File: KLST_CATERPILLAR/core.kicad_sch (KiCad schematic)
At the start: 34 parts, among them SW1 BUTTON_RESET, SW2 BUTTON_BOOT_FLASH, U2 STM32H723ZGTx, Y1 16MHz

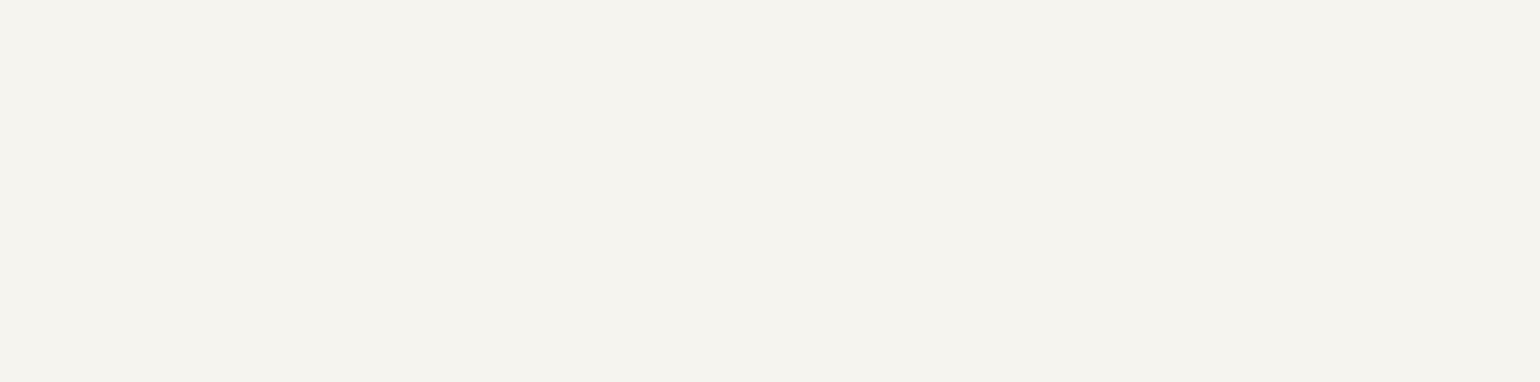
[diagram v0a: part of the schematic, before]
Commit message: reduced modules
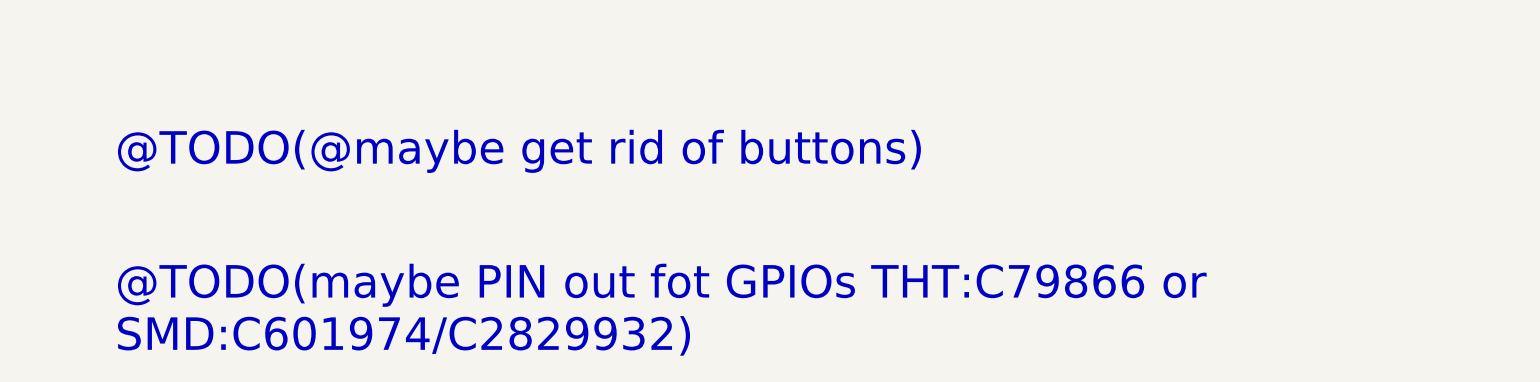
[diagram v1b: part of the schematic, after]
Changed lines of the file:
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@@
+		)
+	)
+	(text_box "@TODO(@maybe get rid of buttons)"
+		(exclude_from_sim no)
+		(at 187.96 186.69 0)
+		(size 201.295 14.605)
+		(stroke
+			(width -0.0001)
+			(type default)
+		)
+		(fill
+			(type color)
+			(color 255 0 0 1)
+		)
+		(effects
+			(font
+				(size 5.08 5.08)
+			)
+			(justify left top)
 		)
 	)
@@
 			)
 			(justify left top)
+		)
+	)
+	(text_box "@TODO(maybe PIN out fot GPIOs THT:C79866 or SMD:C601974/C2829932)"
+		(exclude_from_sim no)
+		(at 187.96 207.645 0)
+		(size 202.565 34.925)
+		(stroke
+			(width -0.0001)
+			(type default)
+		)
+		(fill
+			(type color)
+			(color 255 0 0 1)
+		)
+		(effects
+			(font
+				(size 5.08 5.08)
+			)
+			(justify left top)
